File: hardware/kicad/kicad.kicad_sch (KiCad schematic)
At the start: 31 parts, among them J1 Conn_01x05, J2 USB_C_Receptacle_USB2.0, SW1 SW_Push, U1 RP2040, U2 W25Q128JVS, U3 XC6206PxxxMR, U4 USBLC6-2SC6, Y1 Crystal_GND24_Small

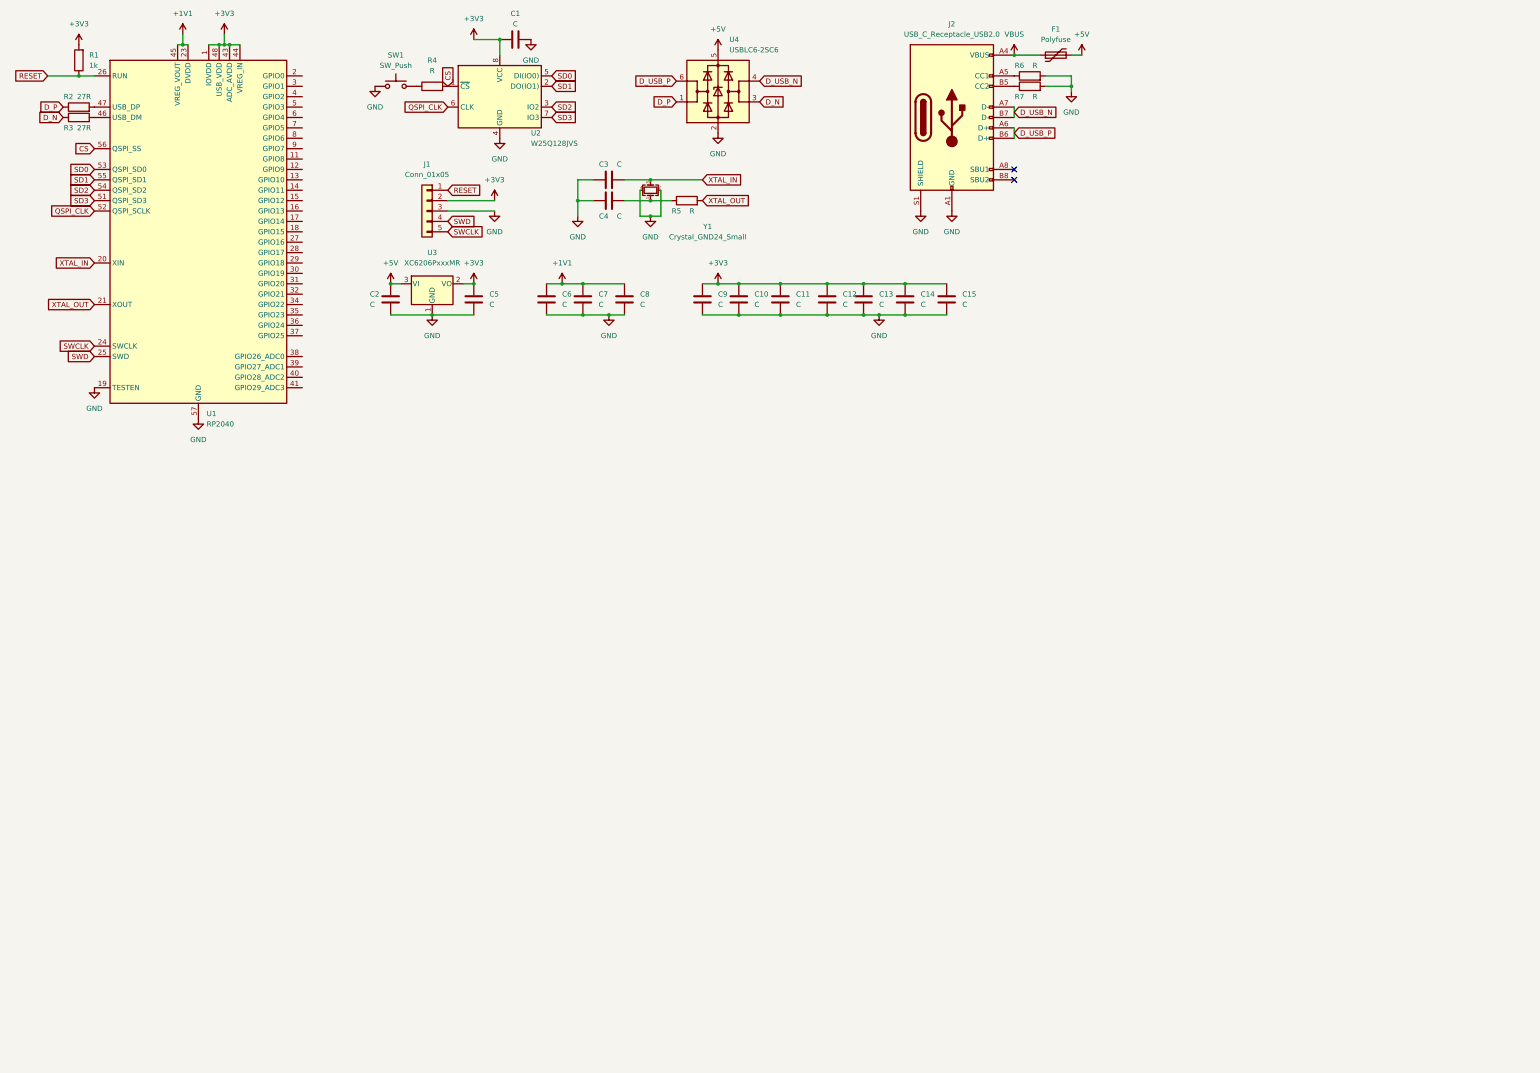
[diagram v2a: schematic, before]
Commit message: [16-09] added level shifter + progress on the expasion connector
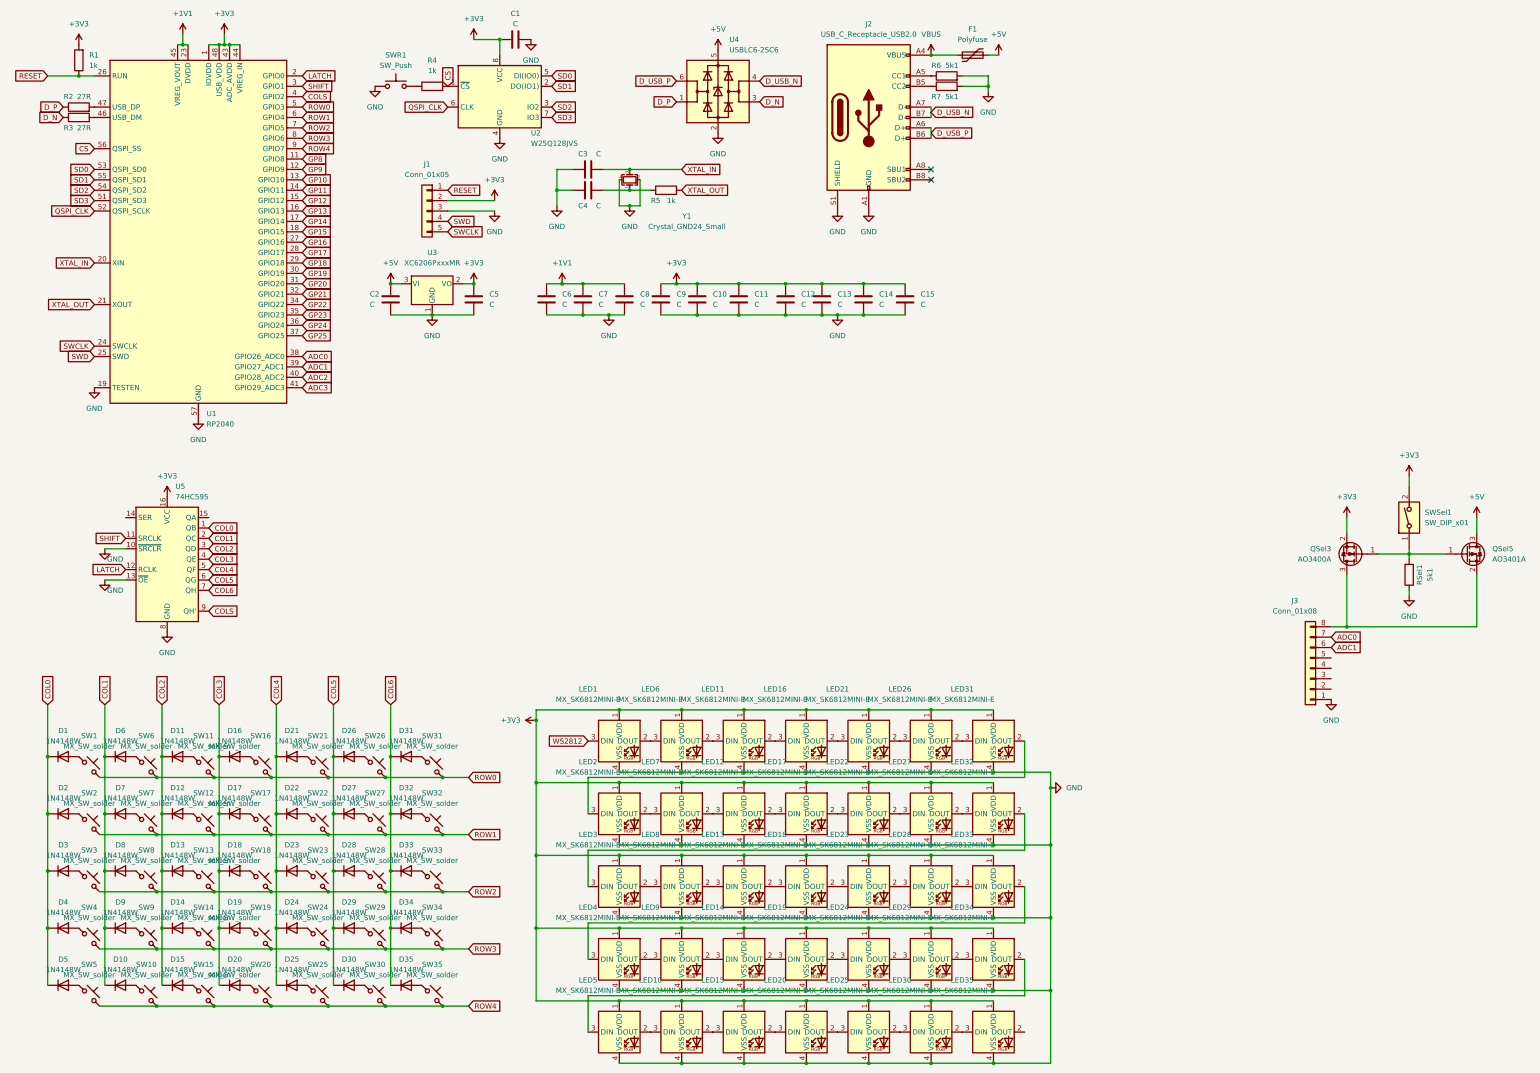
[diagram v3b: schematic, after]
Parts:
- added D1, D10, D11, D12, D13, D14, D15, D16, D17, D18, D19, D2, D20, D21, D22, D23, D24, D25, D26, D27, D28, D29, D3, D30, D31, D32, D33, D34, D35, D4, D5, D6, D7, D8, D9: 1N4148W, Diode_SMD:D_SOD-123, symbol Diode:1N4148W
- added J3: Conn_01x08, Connector_PinHeader_2.54mm:PinHeader_1x08_P2.54mm_Vertical_SMD_Pin1Right, symbol Connector_Generic:Conn_01x08
- added LED1, LED10, LED11, LED12, LED13, LED14, LED15, LED16, LED17, LED18, LED19, LED2, LED20, LED21, LED22, LED23, LED24, LED25, LED26, LED27, LED28, LED29, LED3, LED30, LED31, LED32, LED33, LED34, LED35, LED4, LED5, LED6, LED7, LED8, LED9: MX_SK6812MINI-E, marbastlib-mx:LED_MX_6028R, symbol marbastlib-mx:MX_SK6812MINI-E
- added QSel3: AO3400A, Package_TO_SOT_SMD:SOT-23, symbol Transistor_FET:AO3400A
- added QSel5: AO3401A, Package_TO_SOT_SMD:SOT-23, symbol Transistor_FET:AO3401A
- added RSel1: 5k1, Resistor_SMD:R_0603_1608Metric_Pad0.98x0.95mm_HandSolder, symbol Device:R
- added SW1, SW10, SW11, SW12, SW13, SW14, SW15, SW16, SW17, SW18, SW19, SW2, SW20, SW21, SW22, SW23, SW24, SW25, SW26, SW27, SW28, SW29, SW3, SW30, SW31, SW32, SW33, SW34, SW35, SW4, SW5, SW6, SW7, SW8, SW9: MX_SW_solder, marbastlib-mx:SW_MX_1u, symbol marbastlib-mx:MX_SW_solder
- added SWSel1: SW_DIP_x01, Button_Switch_SMD:SW_DIP_SPSTx01_Slide_6.7x4.1mm_W6.73mm_P2.54mm_LowProfile_JPin, symbol Switch:SW_DIP_x01
- added U5: 74HC595, soic:SOIC16, symbol 74xx:74HC595
- R4, R5: value R -> 1k
- R6, R7: value R -> 5k1
- renumbered SW1 to SWR1
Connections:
- net +3V3: now also LED1.1 (VDD), LED10.1 (VDD), LED11.1 (VDD), LED12.1 (VDD), LED13.1 (VDD), LED14.1 (VDD), LED15.1 (VDD), LED16.1 (VDD), LED17.1 (VDD), LED18.1 (VDD), LED19.1 (VDD), LED2.1 (VDD), LED20.1 (VDD), LED21.1 (VDD), LED22.1 (VDD), LED23.1 (VDD), LED24.1 (VDD), LED25.1 (VDD), LED26.1 (VDD), LED27.1 (VDD), LED28.1 (VDD), LED29.1 (VDD), LED3.1 (VDD), LED30.1 (VDD), LED31.1 (VDD), LED32.1 (VDD), LED33.1 (VDD), LED34.1 (VDD), LED35.1 (VDD), LED4.1 (VDD), LED5.1 (VDD), LED6.1 (VDD), LED7.1 (VDD), LED8.1 (VDD), LED9.1 (VDD), QSel3.2 (S), SWSel1.2, U5.16 (VCC)
- net +5V: now also QSel5.3 (D)
- net GND: now also J3.1 (Pin_1), LED1.4 (VSS), LED10.4 (VSS), LED11.4 (VSS), LED12.4 (VSS), LED13.4 (VSS), LED14.4 (VSS), LED15.4 (VSS), LED16.4 (VSS), LED17.4 (VSS), LED18.4 (VSS), LED19.4 (VSS), LED2.4 (VSS), LED20.4 (VSS), LED21.4 (VSS), LED22.4 (VSS), LED23.4 (VSS), LED24.4 (VSS), LED25.4 (VSS), LED26.4 (VSS), LED27.4 (VSS), LED28.4 (VSS), LED29.4 (VSS), LED3.4 (VSS), LED30.4 (VSS), LED31.4 (VSS), LED32.4 (VSS), LED33.4 (VSS), LED34.4 (VSS), LED35.4 (VSS), LED4.4 (VSS), LED5.4 (VSS), LED6.4 (VSS), LED7.4 (VSS), LED8.4 (VSS), LED9.4 (VSS), RSel1.1, U5.10 (~{SRCLR}), U5.13 (~{OE}), U5.8 (GND)
- net GP8: now reaches U1.11 (GPIO8)
- net GP9: now reaches U1.12 (GPIO9)
- net GP10: now reaches U1.13 (GPIO10)
- net GP11: now reaches U1.14 (GPIO11)
- net GP12: now reaches U1.15 (GPIO12)
- net GP13: now reaches U1.16 (GPIO13)
- net GP14: now reaches U1.17 (GPIO14)
- net GP15: now reaches U1.18 (GPIO15)
- net LATCH: now reaches U1.2 (GPIO0)
- net LATCH: now also U5.12 (RCLK)
- net GP16: now reaches U1.27 (GPIO16)
- net GP17: now reaches U1.28 (GPIO17)
- net GP18: now reaches U1.29 (GPIO18)
- net SHIFT: now reaches U1.3 (GPIO1)
- net SHIFT: now also U5.11 (SRCLK)
- net GP19: now reaches U1.30 (GPIO19)
- net GP20: now reaches U1.31 (GPIO20)
- net GP21: now reaches U1.32 (GPIO21)
- net GP22: now reaches U1.34 (GPIO22)
- net GP23: now reaches U1.35 (GPIO23)
- net GP24: now reaches U1.36 (GPIO24)
- net GP25: now reaches U1.37 (GPIO25)
- net ADC0: now reaches U1.38 (GPIO26_ADC0)
- net ADC0: now also J3.7 (Pin_7)
- net ADC1: now reaches U1.39 (GPIO27_ADC1)
- net ADC1: now also J3.6 (Pin_6)
- net COLS: now reaches U1.4 (GPIO2)
- net COLS: now also U5.9 (QH')
- net ADC2: now reaches U1.40 (GPIO28_ADC2)
- net ADC3: now reaches U1.41 (GPIO29_ADC3)
- net ROW0: now reaches U1.5 (GPIO3)
- net ROW0: now also SW1.2, SW11.2, SW16.2, SW21.2, SW26.2, SW31.2, SW6.2
- net ROW1: now reaches U1.6 (GPIO4)
- net ROW1: now also SW12.2, SW17.2, SW2.2, SW22.2, SW27.2, SW32.2, SW7.2
- net ROW2: now reaches U1.7 (GPIO5)
- net ROW2: now also SW13.2, SW18.2, SW23.2, SW28.2, SW3.2, SW33.2, SW8.2
- net ROW3: now reaches U1.8 (GPIO6)
- net ROW3: now also SW14.2, SW19.2, SW24.2, SW29.2, SW34.2, SW4.2, SW9.2
- net ROW4: now reaches U1.9 (GPIO7)
- net ROW4: now also SW10.2, SW15.2, SW20.2, SW25.2, SW30.2, SW35.2, SW5.2
- new net: LED11.3 (DIN), LED6.2 (DOUT)
- new net: LED1.2 (DOUT), LED6.3 (DIN)
- new net: D20.2 (A), SW20.1
- new net: D31.2 (A), SW31.1
- new net: D13.2 (A), SW13.1
- new net: QSel3.1 (G), QSel5.1 (G), RSel1.2, SWSel1.1
- new net: J3.8 (Pin_8), QSel3.3 (D), QSel5.2 (S)
- new net: D19.2 (A), SW19.1
- new net: LED2.2 (DOUT), LED7.3 (DIN)
- new net: LED2.3 (DIN), LED31.2 (DOUT)
- new net: LED17.2 (DOUT), LED22.3 (DIN)
- new net: LED12.2 (DOUT), LED17.3 (DIN)
- new net: D11.2 (A), SW11.1
- new net: D3.2 (A), SW3.1
- new net: D25.2 (A), SW25.1
- new net: LED18.2 (DOUT), LED23.3 (DIN)
- new net: LED13.2 (DOUT), LED18.3 (DIN)
- new net: D14.2 (A), SW14.1
- new net: D16.2 (A), SW16.1
- new net: LED30.2 (DOUT), LED35.3 (DIN)
- new net: LED23.2 (DOUT), LED28.3 (DIN)
- new net: D6.2 (A), SW6.1
- new net: LED29.2 (DOUT), LED34.3 (DIN)
- new net: LED24.2 (DOUT), LED29.3 (DIN)
- new net: D30.2 (A), SW30.1
- new net: D4.2 (A), SW4.1
- new net: LED21.2 (DOUT), LED26.3 (DIN)
- new net: LED16.2 (DOUT), LED21.3 (DIN)
- new net: D33.2 (A), SW33.1
- new net: LED33.2 (DOUT), LED4.3 (DIN)
- new net: LED28.2 (DOUT), LED33.3 (DIN)
- new net: D17.2 (A), SW17.1
- new net: LED26.2 (DOUT), LED31.3 (DIN)
- new net: D1.2 (A), SW1.1
- new net: D22.2 (A), SW22.1
- new net: LED25.2 (DOUT), LED30.3 (DIN)
- new net: LED20.2 (DOUT), LED25.3 (DIN)
- new net: LED22.2 (DOUT), LED27.3 (DIN)
- new net: D28.2 (A), SW28.1
- new net: D8.2 (A), SW8.1
- new net: D10.2 (A), SW10.1
- new net: LED10.2 (DOUT), LED15.3 (DIN)
- new net: LED10.3 (DIN), LED5.2 (DOUT)
- new net: D26.2 (A), SW26.1
- new net: D35.2 (A), SW35.1
- new net: LED14.2 (DOUT), LED19.3 (DIN)
- new net: LED14.3 (DIN), LED9.2 (DOUT)
- new net: D21.2 (A), SW21.1
- new net: D9.2 (A), SW9.1
- new net: D34.2 (A), SW34.1
- new net: D2.2 (A), SW2.1
- new net: D27.2 (A), SW27.1
- new net: LED15.2 (DOUT), LED20.3 (DIN)
- new net: LED12.3 (DIN), LED7.2 (DOUT)
- new net: LED3.3 (DIN), LED32.2 (DOUT)
- new net: LED27.2 (DOUT), LED32.3 (DIN)
- new net: D24.2 (A), SW24.1
- new net: D18.2 (A), SW18.1
- new net: D15.2 (A), SW15.1
- new net: LED13.3 (DIN), LED8.2 (DOUT)
- new net: LED3.2 (DOUT), LED8.3 (DIN)
- new net: D12.2 (A), SW12.1
- new net: D32.2 (A), SW32.1
- new net: D23.2 (A), SW23.1
- new net: LED19.2 (DOUT), LED24.3 (DIN)
- new net: LED4.2 (DOUT), LED9.3 (DIN)
- new net: D7.2 (A), SW7.1
- new net: LED34.2 (DOUT), LED5.3 (DIN)
- new net: LED11.2 (DOUT), LED16.3 (DIN)
- new net: D29.2 (A), SW29.1
- new net: D5.2 (A), SW5.1
- new net COL0: D1.1 (K), D2.1 (K), D3.1 (K), D4.1 (K), D5.1 (K), U5.1 (QB)
- new net COL1: D10.1 (K), D6.1 (K), D7.1 (K), D8.1 (K), D9.1 (K), U5.2 (QC)
- new net COL2: D11.1 (K), D12.1 (K), D13.1 (K), D14.1 (K), D15.1 (K), U5.3 (QD)
- new net COL3: D16.1 (K), D17.1 (K), D18.1 (K), D19.1 (K), D20.1 (K), U5.4 (QE)
- new net COL4: D21.1 (K), D22.1 (K), D23.1 (K), D24.1 (K), D25.1 (K), U5.5 (QF)
- new net COL5: D26.1 (K), D27.1 (K), D28.1 (K), D29.1 (K), D30.1 (K), U5.6 (QG)
- new net COL6: D31.1 (K), D32.1 (K), D33.1 (K), D34.1 (K), D35.1 (K), U5.7 (QH)
- new net WS2812: LED1.3 (DIN)
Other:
- moved on the sheet: C10, C11, C12, C13, C14, C15, C3, C4, C9, F1, J2, R5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
